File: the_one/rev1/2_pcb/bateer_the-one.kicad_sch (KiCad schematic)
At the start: 0 parts

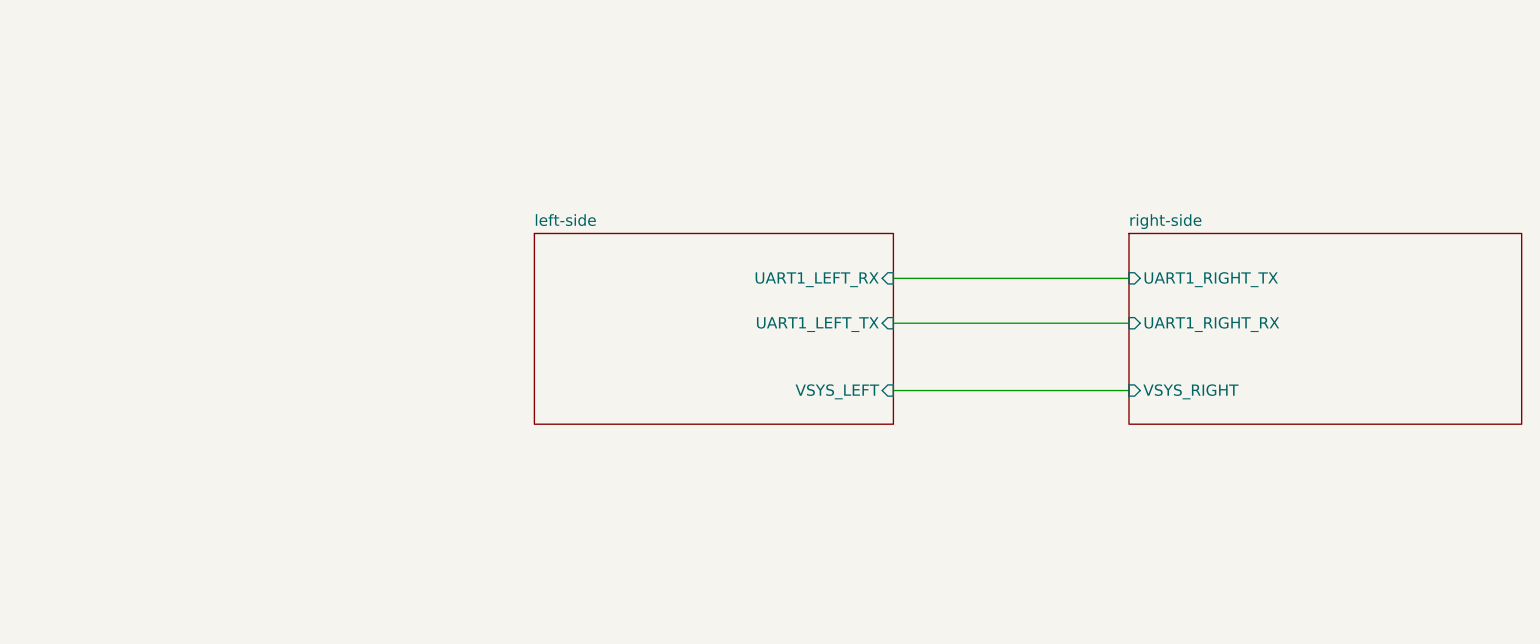
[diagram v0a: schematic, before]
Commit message: update KiCAD schematcis
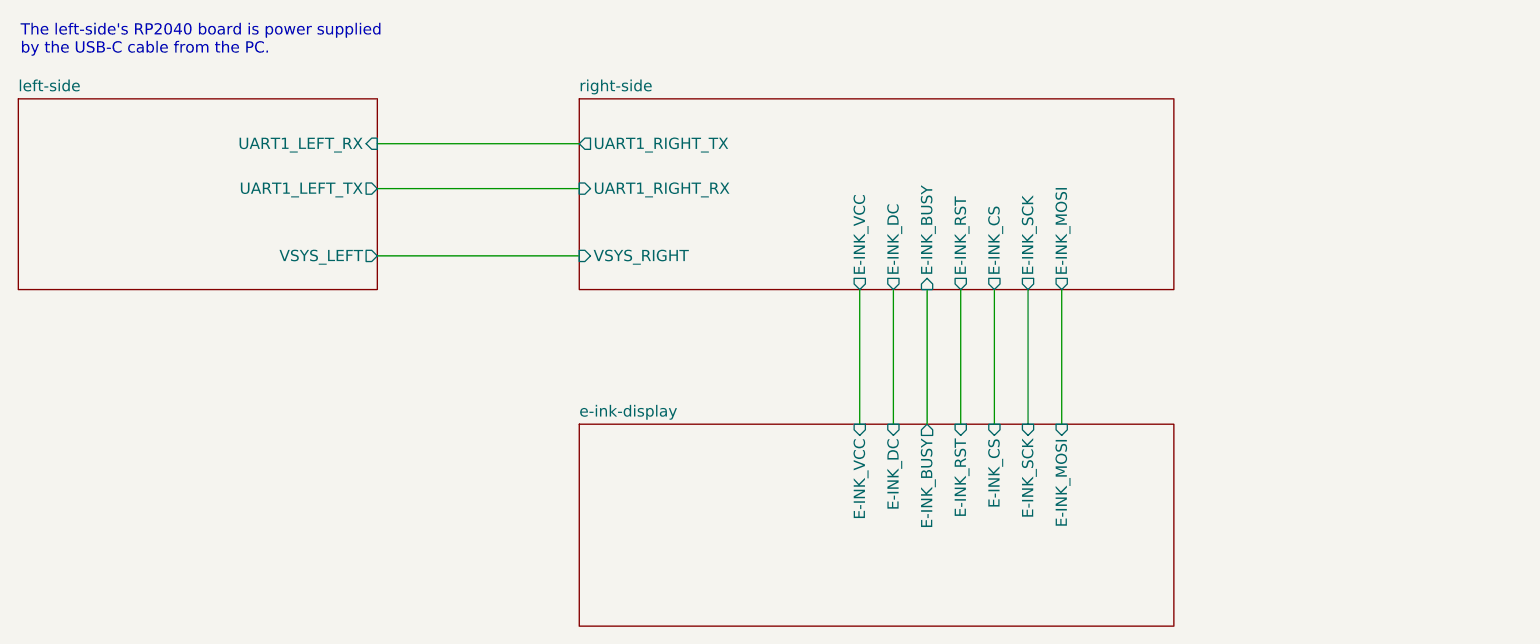
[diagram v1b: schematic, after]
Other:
- added sheet e-ink-display (e-ink-display.kicad_sch)
- sheet right-side ports: added E-INK_BUSY, E-INK_CS, E-INK_DC, E-INK_MOSI, E-INK_RST, E-INK_SCK, E-INK_VCC; removed none
- note added: "The left-side's RP2040 board is power supplied by the USB-C cable from the PC."
